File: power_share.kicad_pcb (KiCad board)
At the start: 2 copper layers, 32.5 x 21.1 mm, 22 parts, among them J1 Conn_01x02, J2 Conn_01x03, Q1 NX3008NBKW, Q2 NX3008NBKW, U1 LTC4370

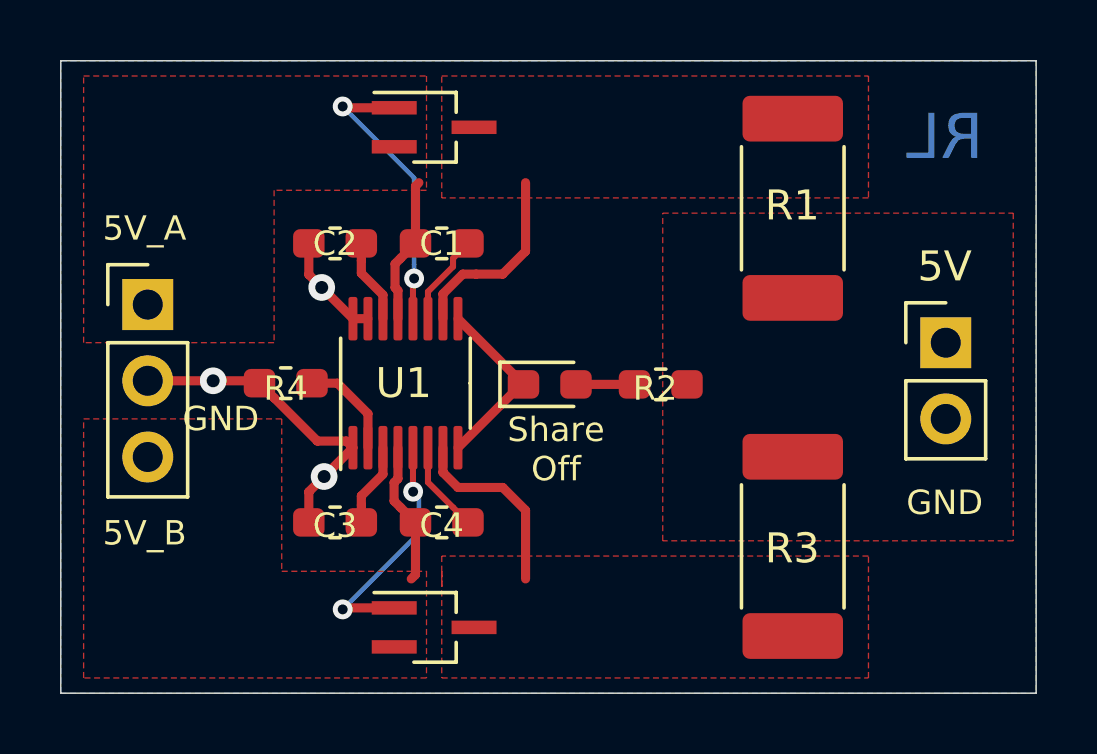
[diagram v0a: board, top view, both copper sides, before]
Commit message: tighten up board
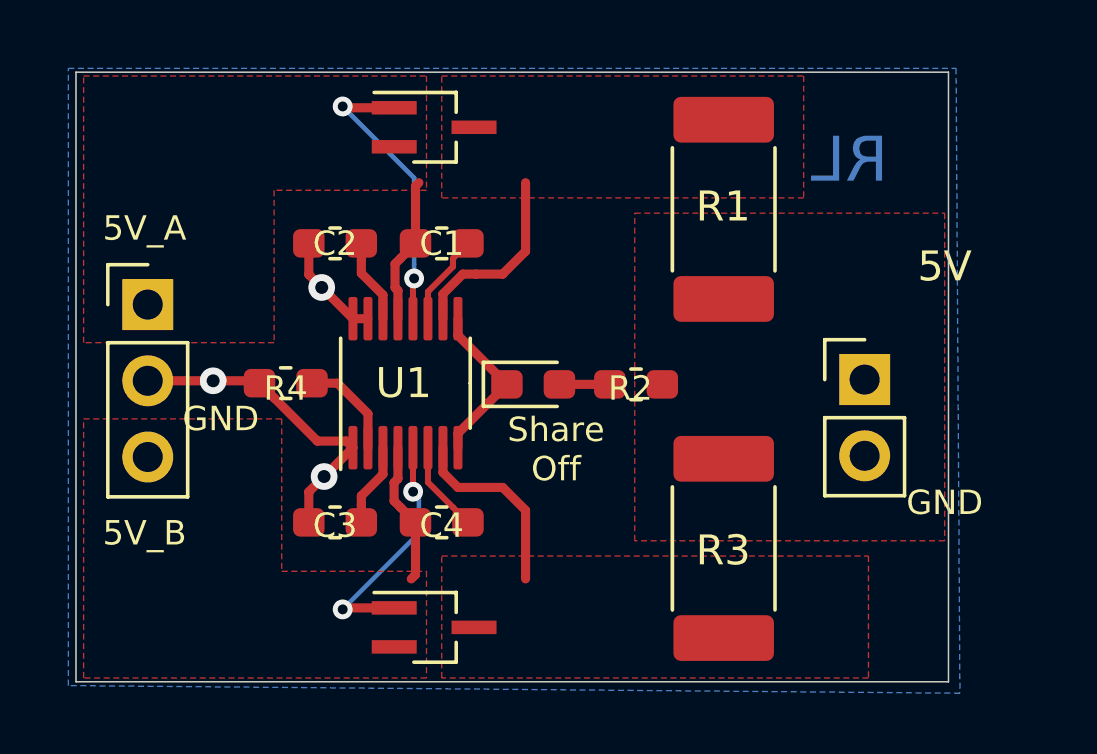
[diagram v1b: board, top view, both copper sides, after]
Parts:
- moved J1 2.97 mm to (141.1, 93.9)
- moved R3 2.30 mm to (136.4, 99.6)
- moved R1 2.30 mm to (136.4, 88.3)
- moved R2 0.82 mm to (133.5, 94.1)
- moved G*** 0.65 mm to (129.9, 93.3)
- moved D1 0.55 mm to (130.0, 94.1)
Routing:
- net Net-(D1-Pad1): track 6.15 -> 5.65 mm
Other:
- board size 32.5 x 21.1 mm -> 29.1 x 20.3 mm
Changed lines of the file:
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@@
   )
   (setup
-    (last_trace_width 0.1524)
+    (last_trace_width 0.3048)
     (user_trace_width 0.2032)
     (user_trace_width 0.3048)
@@
   )
   (module Logos:asian_tiger (layer F.Cu)
-    (at 130.556 93.472)
+    (at 129.921 93.345)
     (attr virtual)
     (fp_text reference G*** (at 0 0) (layer F.SilkS) hide
@@
   )
   (module Connector_PinHeader_2.54mm:PinHeader_1x02_P2.54mm_Vertical (layer F.Cu)
-    (at 143.8 92.71)
+    (at 141.097 93.94)
     (descr "Through hole straight pin header, 1x02, 2.54mm pitch, single row")
     (tags "Through hole pin header THT 1x02 2.54mm single row")
@@
       (effects (font (size 1 1) (thickness 0.15)))
     )
-    (fp_text value Conn_01x02 (at 0 4.87) (layer F.Fab)
+    (fp_text value Conn_01x02 (at -2.159 -2.627) (layer F.Fab)
       (effects (font (size 1 1) (thickness 0.15)))
     )
@@
   )
   (module LED_SMD:LED_0603_1608Metric_Pad1.05x0.95mm_HandSolder (layer F.Cu)
-    (at 130.6 94.1)
+    (at 130.048 94.1)
     (descr "LED SMD 0603 (1608 Metric), square (rectangular) end terminal, IPC_7351 nominal, (Body size source: http://www.tortai-tech.com/upload/download/2011102023233369053.pdf), generated with kicad-footprint-generator")
     (tags "LED handsolder")
@@
   )
   (module Resistor_SMD:R_2512_6332Metric_Pad1.52x3.35mm_HandSolder (layer F.Cu)
-    (at 138.7 99.5 270)
+    (at 136.398 99.568 270)
     (descr "Resistor SMD 2512 (6332 Metric), square (rectangular) end terminal, IPC_7351 nominal with elongated pad for handsoldering. (Body size source: http://www.tortai-tech.com/upload/download/2011102023233369053.pdf), generated with kicad-footprint-generator")
     (tags "resistor handsolder")
@@
   )
   (module Resistor_SMD:R_0603_1608Metric_Pad1.05x0.95mm_HandSolder (layer F.Cu)
-    (at 134.3 94.1 180)
+    (at 133.477 94.1 180)
     (descr "Resistor SMD 0603 (1608 Metric), square (rectangular) end terminal, IPC_7351 nominal with elongated pad for handsoldering. (Body size source: http://www.tortai-tech.com/upload/download/2011102023233369053.pdf), generated with kicad-footprint-generator")
     (tags "resistor handsolder")
@@
   )
   (module Resistor_SMD:R_2512_6332Metric_Pad1.52x3.35mm_HandSolder (layer F.Cu)
-    (at 138.7 88.23 270)
+    (at 136.398 88.265 270)
     (descr "Resistor SMD 2512 (6332 Metric), square (rectangular) end terminal, IPC_7351 nominal with elongated pad for handsoldering. (Body size source: http://www.tortai-tech.com/upload/download/2011102023233369053.pdf), generated with kicad-footprint-generator")
     (tags "resistor handsolder")
@@
     )
   )
-  (gr_text RL (at 143.764 85.852) (layer B.Cu)
+  (gr_text RL (at 140.589 86.614) (layer B.Cu)
     (effects (font (size 1.5 1.5) (thickness 0.3)) (justify mirror))
   )
@@
     (effects (font (size 0.8128 0.8128) (thickness 0.1524)))
   )
-  (gr_line (start 114.3 104.394) (end 114.3 83.312) (layer Edge.Cuts) (width 0.05))
-  (gr_line (start 146.812 104.394) (end 114.3 104.394) (layer Edge.Cuts) (width 0.05))
-  (gr_line (start 146.812 83.312) (end 146.812 104.394) (layer Edge.Cuts) (width 0.05))
-  (gr_line (start 114.3 83.312) (end 146.812 83.312) (layer Edge.Cuts) (width 0.05))
+  (gr_line (start 114.808 104.013) (end 114.808 83.693) (layer Edge.Cuts) (width 0.05))
+  (gr_line (start 143.891 104.013) (end 114.808 104.013) (layer Edge.Cuts) (width 0.05))
+  (gr_line (start 143.891 83.693) (end 143.891 104.013) (layer Edge.Cuts) (width 0.05))
+  (gr_line (start 114.808 83.693) (end 143.891 83.693) (layer Edge.Cuts) (width 0.05))
   (gr_text "Share\nOff" (at 130.81 96.266) (layer F.SilkS)
     (effects (font (size 0.8128 0.8128) (thickness 0.1524)))
@@
   (segment (start 126.04 97.670922) (end 126.046082 97.677004) (width 0.2032) (layer F.Cu) (net 10))
   (via (at 126.046082 97.677004) (size 0.6604) (drill 0.3302) (layers F.Cu B.Cu) (net 10))
-  (segment (start 131.475 94.1) (end 133.425 94.1) (width 0.3048) (layer F.Cu) (net 12))
+  (segment (start 130.923 94.1) (end 132.602 94.1) (width 0.3048) (layer F.Cu) (net 12))
   (segment (start 123.524 94.06) (end 122.675 94.06) (width 0.3048) (layer F.Cu) (net 13))
   (segment (start 124.54 95.076) (end 123.524 94.06) (width 0.3048) (layer F.Cu) (net 13))
   (segment (start 124.54 96.21) (end 124.54 95.076) (width 0.3048) (layer F.Cu) (net 13))
-  (segment (start 129.65 94.1) (end 129.725 94.1) (width 0.3048) (layer F.Cu) (net 14))
-  (segment (start 127.54 96.21) (end 129.65 94.1) (width 0.3048) (layer F.Cu) (net 14))
-  (segment (start 129.725 94.095) (end 129.725 94.1) (width 0.3048) (layer F.Cu) (net 14))
-  (segment (start 127.54 91.91) (end 129.725 94.095) (width 0.3048) (layer F.Cu) (net 14))
+  (segment (start 127.54 92.467) (end 129.173 94.1) (width 0.3048) (layer F.Cu) (net 14))
+  (segment (start 127.54 91.91) (end 127.54 92.467) (width 0.3048) (layer F.Cu) (net 14))
+  (segment (start 127.54 95.733) (end 129.173 94.1) (width 0.3048) (layer F.Cu) (net 14))
+  (segment (start 127.54 96.21) (end 127.54 95.733) (width 0.3048) (layer F.Cu) (net 14))
   (segment (start 127.04 91.085) (end 127.701 90.424) (width 0.3048) (layer F.Cu) (net 15))
   (segment (start 127.04 91.91) (end 127.04 91.085) (width 0.3048) (layer F.Cu) (net 15))
@@
   (segment (start 129.794 89.662) (end 129.794 87.376) (width 0.3048) (layer F.Cu) (net 15))
   (zone (net 11) (net_name 5V) (layer F.Cu) (hatch edge 0.508)
-    (connect_pads (clearance 0.508))
+    (connect_pads yes (clearance 0.508))
     (min_thickness 0.254)
     (fill yes (arc_segments 32) (thermal_gap 0.508) (thermal_bridge_width 0.508))
     (polygon
       (pts
-        (xy 134.366 88.392) (xy 146.05 88.392) (xy 146.05 99.314) (xy 134.366 99.314)
+        (xy 133.43284 88.392) (xy 143.764 88.392) (xy 143.764 99.314) (xy 133.43284 99.314)
       )
     )
   )
   (zone (net 6) (net_name 5V_B) (layer F.Cu) (hatch edge 0.508)
-    (connect_pads (clearance 0.508))
+    (connect_pads yes (clearance 0.508))
     (min_thickness 0.254)
     (fill yes (arc_segments 32) (thermal_gap 0.508) (thermal_bridge_width 0.508))
@@
   )
   (zone (net 2) (net_name 5V_A) (layer F.Cu) (hatch edge 0.508)
-    (connect_pads (clearance 0.508))
+    (connect_pads yes (clearance 0.508))
     (min_thickness 0.254)
     (fill yes (arc_segments 32) (thermal_gap 0.508) (thermal_bridge_width 0.508))
@@
   )
   (zone (net 9) (net_name "Net-(Q2-Pad3)") (layer F.Cu) (hatch edge 0.508)
-    (connect_pads (clearance 0.508))
+    (connect_pads yes (clearance 0.508))
     (min_thickness 0.254)
     (fill yes (arc_segments 32) (thermal_gap 0.508) (thermal_bridge_width 0.508))
     (polygon
       (pts
-        (xy 127 100.33) (xy 127 103.886) (xy 141.224 103.886) (xy 141.224 99.822) (xy 127 99.822)
-        (xy 127 100.838)
+        (xy 141.224 103.886) (xy 127 103.886) (xy 127 99.822) (xy 141.224 99.822)
       )
     )
   )
   (zone (net 15) (net_name "Net-(Q1-Pad3)") (layer F.Cu) (hatch edge 0.508)
-    (connect_pads (clearance 0.508))
+    (connect_pads yes (clearance 0.508))
     (min_thickness 0.254)
     (fill yes (arc_segments 32) (thermal_gap 0.508) (thermal_bridge_width 0.508))
     (polygon
       (pts
-        (xy 127 83.82) (xy 141.224 83.82) (xy 141.224 87.884) (xy 127 87.884)
+        (xy 127 83.82) (xy 139.065 83.82) (xy 139.065 87.884) (xy 127 87.884)
       )
     )
   )
   (zone (net 3) (net_name GND) (layer B.Cu) (hatch edge 0.508)
-    (connect_pads (clearance 0.508))
+    (connect_pads yes (clearance 0.508))
     (min_thickness 0.254)
     (fill yes (arc_segments 32) (thermal_gap 0.508) (thermal_bridge_width 0.508))
     (polygon
       (pts
-        (xy 114.3 83.312) (xy 146.812 83.312) (xy 146.812 104.394) (xy 114.3 104.394)
+        (xy 114.554 83.566) (xy 144.145 83.566) (xy 144.272 104.394) (xy 114.554 104.14)
       )
     )
